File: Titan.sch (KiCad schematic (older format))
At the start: 155 parts, among them J1 USB_B_Micro, J10 PWM1, J11 SPI SLAVE, J12 IO Conn 2, J13 IO Conn 1, J14 ADC EXT, J15 PWM2, J2 USB_B_Micro, J3 Uart 1, J4 Bat Conn, J5 Debug, J6 Uart 2, J7 SPI AUX MASTER, J8 S3B-ZR(LF)(SN), J9 S3B-ZR(LF)(SN), Q1 NDS332P, Q2 NDS332P, SW1 SW_Push, SW2 SW_DPDT_x2, U1 FT230XS, U2 SR10S3V3, U3 STM32F413VGTx, U4 CY15B104Q, U5 MPU-6050, U6 FT230XS, U7 XBEE3Micro, U8 MPU-6050

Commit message: First commit of TitanV2
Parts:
- removed C1, C2: 470uF, Titan:T59EE477M016C0025, symbol 2020-03-08_10-59-35:UCD1E471MNL1GS
- removed D2: PWR_ON, LED_SMD:LED_0805_2012Metric_Pad1.15x1.40mm_HandSolder, symbol Device:LED
- removed J10: PWM1, Footprint:HDRV8W85P254_8X1_2078X650X1000, symbol 282834-8:282834-8
- removed J11: SPI SLAVE, Connector_PinHeader_2.54mm:PinHeader_2x03_P2.54mm_Vertical, symbol Connector_Generic:Conn_02x03_Odd_Even
- removed J12: IO Conn 2, Connector_PinHeader_2.54mm:PinHeader_2x05_P2.54mm_Vertical, symbol Connector_Generic:Conn_02x05_Top_Bottom
- removed J13: IO Conn 1, Connector_PinHeader_2.54mm:PinHeader_2x07_P2.54mm_Vertical, symbol Connector_Generic:Conn_02x07_Top_Bottom
- removed J14: ADC EXT, Connector_PinHeader_2.54mm:PinHeader_2x03_P2.54mm_Vertical, symbol Connector_Generic:Conn_02x03_Odd_Even
- removed J15: PWM2, Footprint:HDRV8W85P254_8X1_2078X650X1000, symbol 282834-8:282834-8
- removed J4: Bat Conn, digikey-footprints:Terminal_Block_D1.3mm_P5mm, symbol dk_Terminal-Blocks-Wire-to-Board:1935161
- removed J6: Uart 2, TerminalBlock_TE-Connectivity:TerminalBlock_TE_282834-4_1x04_P2.54mm_Horizontal, symbol Connector:Screw_Terminal_01x04
- removed J7: SPI AUX MASTER, Connector_PinHeader_2.54mm:PinHeader_2x03_P2.54mm_Vertical, symbol Connector_Generic:Conn_02x03_Odd_Even
- removed L1: 1231AS-H-6R4M=P3, Footprint:IND_1231AS-H-6R4M=P3, symbol 1231AS-H-6R4M_P3:1231AS-H-6R4M=P3
- removed R1: 330, Resistor_SMD:R_0603_1608Metric_Pad1.05x0.95mm_HandSolder, symbol Device:R
- removed R16, R17, R19, R39, R40, R41, R42, R8: 220, Resistor_SMD:R_0603_1608Metric_Pad1.05x0.95mm_HandSolder, symbol Device:R
- removed R18, R63, R7: 0, Resistor_SMD:R_0603_1608Metric_Pad1.05x0.95mm_HandSolder, symbol Device:R
- removed R4, R5: 10k, Resistor_SMD:R_0603_1608Metric_Pad1.05x0.95mm_HandSolder, symbol Device:R
- removed R43, R44, R45, R46, R47, R48, R49, R50, R51, R52, R53, R54, R55, R56, R57, R58: 1K, Resistor_SMD:R_0603_1608Metric_Pad1.05x0.95mm_HandSolder, symbol Device:R_Small
- removed SW1: SW_Push, Titan:TL3301AF160QG, symbol Switch:SW_Push
- removed SW2: SW_DPDT_x2, Titan:CASD20, symbol Switch:SW_DPDT_x2
- removed TP1, TP2: TestPoint, TestPoint:TestPoint_Pad_1.5x1.5mm, symbol Connector:TestPoint
- removed U2: SR10S3V3, Titan:SR10S3V3, symbol TitanCustom:SR10S3V3
- added C1: 2.2uF, Capacitor_SMD:C_0603_1608Metric_Pad1.08x0.95mm_HandSolder, symbol Device:C
- added D2: D_Schottky, Diode_SMD:D_SOD-123, symbol Device:D_Schottky
- added J4: Screw_Terminal_01x08, Footprint:HDRV8W85P254_8X1_2078X650X1000, symbol Connector:Screw_Terminal_01x08
- added S1: Reset button, digikey-footprints:Switch_Tactile_SMD_4.5x4.5mm_TL3315NF160Q, symbol dk_Tactile-Switches:TL3315NF160Q
- added U2: ST730M33R, Package_TO_SOT_SMD:SOT-23-5_HandSoldering, symbol TitanCustom:ST730M33R
- C10, C11, C12, C13, C14, C15, C16, C17, C18, C19, C20, C21, C22, C23, C24, C25, C26, C27, C28, C29, C3, C30, C31, C32, C33, C35, C36, C4, C5, C55, C56, C6, C7, C8, C9: footprint Capacitor_SMD:C_0603_1608Metric_Pad1.05x0.95mm_HandSolder -> Capacitor_SMD:C_0603_1608Metric_Pad1.08x0.95mm_HandSolder
- C34: value 22uF -> 2.2uF; footprint Capacitor_SMD:C_0603_1608Metric_Pad1.05x0.95mm_HandSolder -> Capacitor_SMD:C_0603_1608Metric_Pad1.08x0.95mm_HandSolder
- FB1: footprint Resistor_SMD:R_0805_2012Metric_Pad1.15x1.40mm_HandSolder -> Resistor_SMD:R_0805_2012Metric_Pad1.20x1.40mm_HandSolder
- J1, J2: symbol Connector:USB_B_Micro -> Titan-rescue:USB_B_Micro-Connector
- J3: value Uart 1 -> PWR CON
- Q1, Q2: footprint digikey-footprints:SOT-23-3 -> Titan:SOT-23-3
- R10, R11, R12, R13, R14, R15, R2, R20, R21, R22, R23, R24, R25, R26, R27, R28, R29, R3, R30, R31, R32, R33, R34, R35, R36, R37, R38, R59, R6, R60, R61, R62, R68, R69, R70, R71, R72, R9: footprint Resistor_SMD:R_0603_1608Metric_Pad1.05x0.95mm_HandSolder -> Resistor_SMD:R_0603_1608Metric_Pad0.98x0.95mm_HandSolder
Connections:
- net labels added: VBUS_COM
- net labels removed: ADC_1, ADC_2, ADC_3, BOOT0, IO_1, IO_10, IO_11, IO_12, IO_13, IO_14, IO_15, IO_16, IO_2, IO_3, IO_4, IO_5, IO_6, IO_7, IO_8, IO_9, IO_CON_1, IO_CON_10, IO_CON_11, IO_CON_12, IO_CON_13, IO_CON_14, IO_CON_15, IO_CON_16, IO_CON_2, IO_CON_3, IO_CON_4, IO_CON_5, IO_CON_6, IO_CON_7, IO_CON_8, IO_CON_9, SPI_AUX_MISO, SPI_AUX_MOSI, SPI_AUX_NSS, SPI_AUX_SCK, SPI_SLAVE_MISO, SPI_SLAVE_MOSI, SPI_SLAVE_NSS, SPI_SLAVE_SCK, UART_MOTOR_1_RX, UART_MOTOR_1_TX
- wire segments 617 -> 453
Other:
- note added: "Revision 1 of titan."
- note removed: "Boot config"
- note removed: "Motor control connectors"
- moved on the sheet: C10, C12, C13, C18, C19, C23, C24, C25, C26, C27, C28, C3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

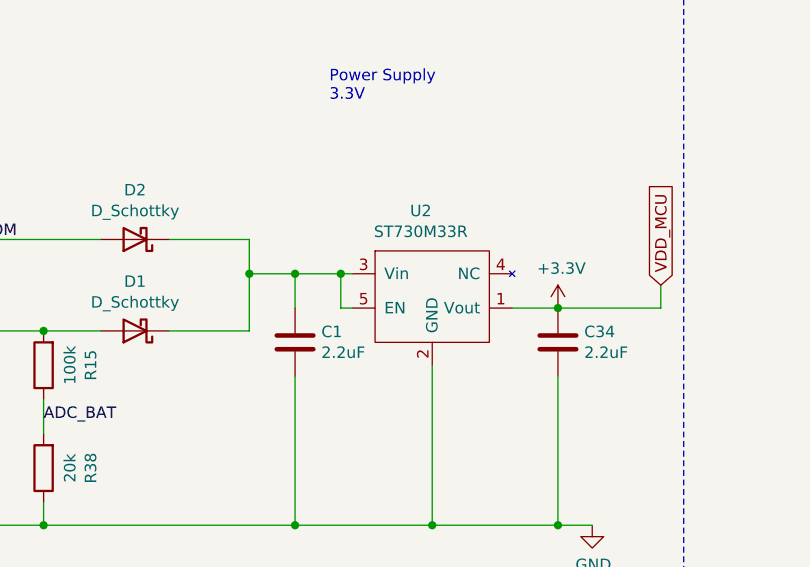
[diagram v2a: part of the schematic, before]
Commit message: As ordered from Aisler.
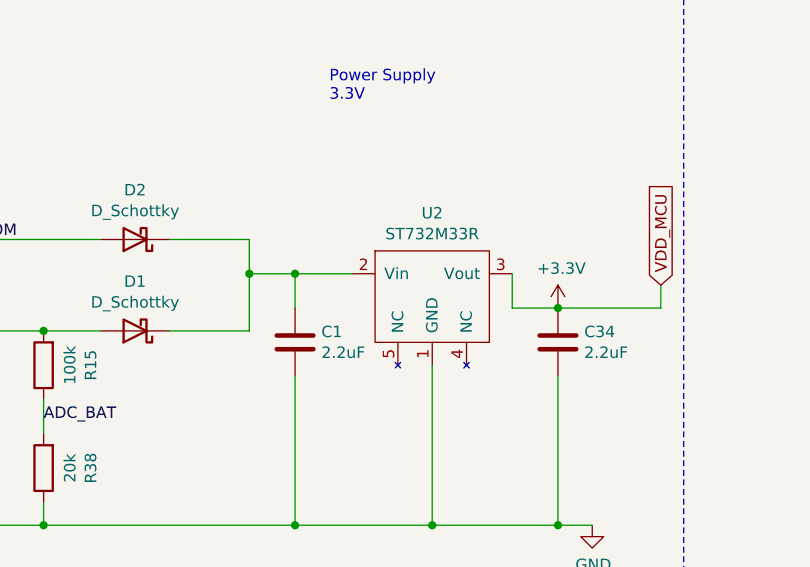
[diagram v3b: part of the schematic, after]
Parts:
- removed U2: ST730M33R, Package_TO_SOT_SMD:SOT-23-5_HandSoldering, symbol TitanCustom:ST730M33R
- added U2: ST732M33R, Package_TO_SOT_SMD:SOT-23-5_HandSoldering, symbol TitanCustom:ST732M33R
- S1: footprint digikey-footprints:Switch_Tactile_SMD_4.5x4.5mm_TL3315NF160Q -> digikey-footprints:Switch_Tactile_SMD_6x6mm
- U4: footprint Footprint:SOIC127P523X800X203-8N -> Package_SO:SOP-8_3.9x4.9mm_P1.27mm
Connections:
- net +3V3: now also U2.3 (Vout)
- net GND: now also U2.1 (GND)
- net at C1.1, D1.1 (K), D2.1 (K): now also U2.2 (Vin)
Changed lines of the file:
@@
 F 0 "U4" H 16150 5775 50  0000 C CNN
 F 1 "CY15B104Q" H 16150 5684 50  0000 C CNN
-F 2 "Footprint:SOIC127P523X800X203-8N" H 16150 5650 50  0001 C CNN
+F 2 "Package_SO:SOP-8_3.9x4.9mm_P1.27mm" H 16150 5650 50  0001 C CNN
 F 3 "" H 16150 5650 50  0001 C CNN
 	1    16150 5650
@@
 F 0 "S1" H 10200 5297 60  0000 C CNN
 F 1 "Reset button" H 10200 5191 60  0000 C CNN
-F 2 "digikey-footprints:Switch_Tactile_SMD_4.5x4.5mm_TL3315NF160Q" H 10400 5150 60  0001 L CNN
+F 2 "digikey-footprints:Switch_Tactile_SMD_6x6mm" H 10400 5150 60  0001 L CNN
 F 3 "http://spec_sheets.e-switch.com/specs/P010337.pdf" H 10400 5250 60  0001 L CNN
 F 4 "EG4621CT-ND" H 10400 5350 60  0001 L CNN "Digi-Key_PN"
@@
 Text Label 14550 13450 0    50   ~ 0
 PWM_2
-$Comp
-L TitanCustom:ST730M33R U2
-U 1 1 643D46A2
-P 4800 2300
-F 0 "U2" H 4750 2525 50  0000 C CNN
-F 1 "ST730M33R" H 4750 2434 50  0000 C CNN
-F 2 "Package_TO_SOT_SMD:SOT-23-5_HandSoldering" H 4800 2300 50  0001 C CNN
-F 3 "" H 4800 2300 50  0001 C CNN
-	1    4800 2300
-	1    0    0    -1
-$EndComp
 Wire Wire Line
 	5800 2400 5800 2500
-Wire Wire Line
-	4450 2350 4400 2350
-Wire Wire Line
-	4450 2500 4400 2500
-Wire Wire Line
-	4400 2500 4400 2350
-Connection ~ 4400 2350
 Wire Wire Line
 	4800 2750 4800 3450
@@
 Connection ~ 4200 2350
 Wire Wire Line
-	4200 2350 4400 2350
-Wire Wire Line
 	4200 2800 4200 3450
 Connection ~ 4200 3450
@@
 VBUS_COM
 Connection ~ 1700 8400
+$Comp
+L TitanCustom:ST732M33R U2
+U 1 1 604346A5
+P 4800 2300
+F 0 "U2" H 4800 2515 50  0000 C CNN
+F 1 "ST732M33R" H 4800 2424 50  0000 C CNN
+F 2 "Package_TO_SOT_SMD:SOT-23-5_HandSoldering" H 4800 2300 50  0001 C CNN
+F 3 "" H 4800 2300 50  0001 C CNN
+	1    4800 2300
+	1    0    0    -1
+$EndComp
+Wire Wire Line
+	4200 2350 4450 2350
+Wire Wire Line
+	5150 2500 5150 2350
 $EndSCHEMATC
